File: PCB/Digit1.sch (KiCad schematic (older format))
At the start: 29 parts

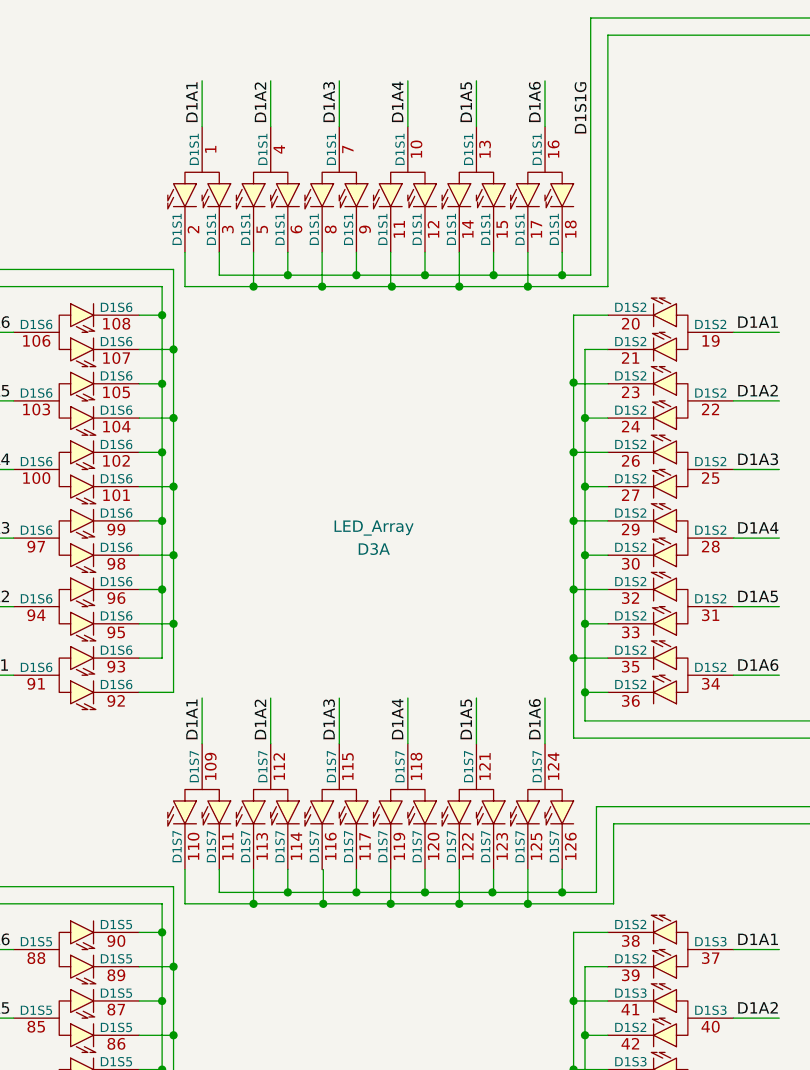
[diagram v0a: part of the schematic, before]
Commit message: Updated schematic.
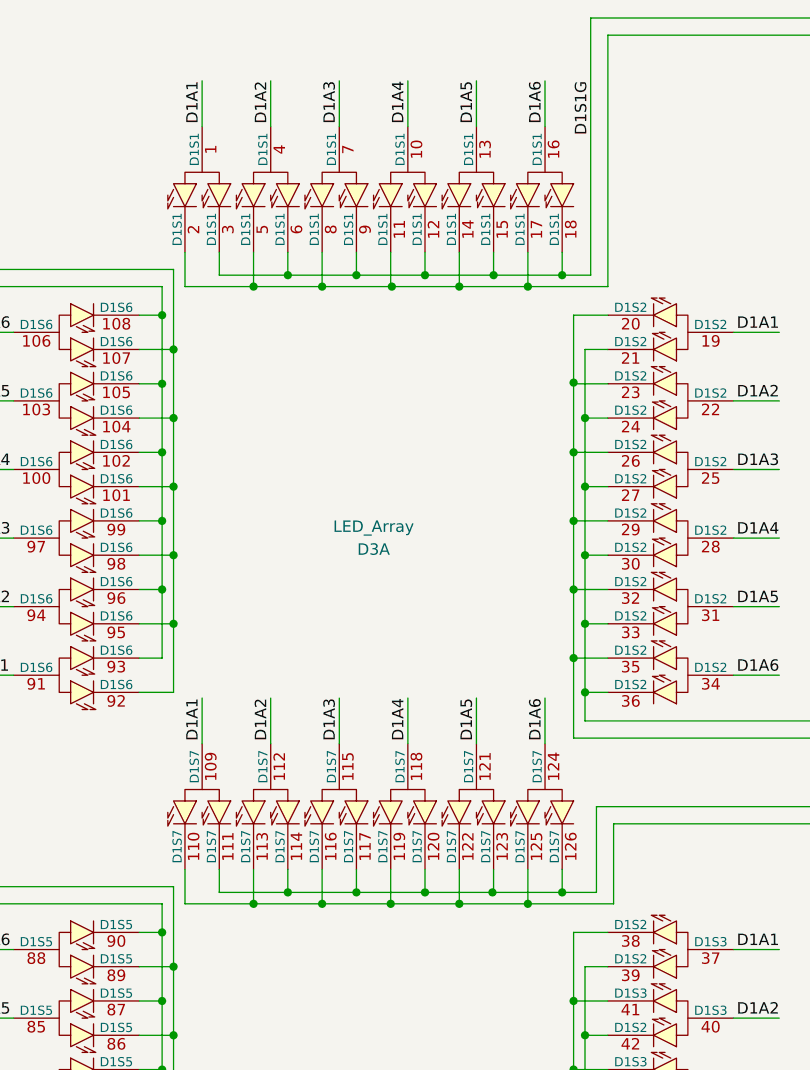
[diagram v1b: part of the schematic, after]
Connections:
- net at D3.110 (D1S7), D3.113 (D1S7), D3.119 (D1S7)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: now also D3.116 (D1S7)
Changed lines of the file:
@@
 Connection ~ 3930 4550
-Wire Wire Line
-	4235 4400 4235 4550
-Connection ~ 4235 4550
 Wire Wire Line
 	4530 4400 4530 4550
@@
 	3780 1700 3780 1800
 Wire Wire Line
-	5405 1800 3780 1800
-Wire Wire Line
-	5405 675  5405 1800
+	3780 1800 5405 1800
+Wire Wire Line
+	5405 1800 5405 675
 Wire Wire Line
 	3930 1700 3930 1850
@@
 Wire Wire Line
 	5405 675  8800 675
+Wire Wire Line
+	4230 4400 4230 4550
+Connection ~ 4230 4550
 $EndSCHEMATC
